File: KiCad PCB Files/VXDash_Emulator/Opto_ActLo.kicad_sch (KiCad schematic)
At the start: 3 parts

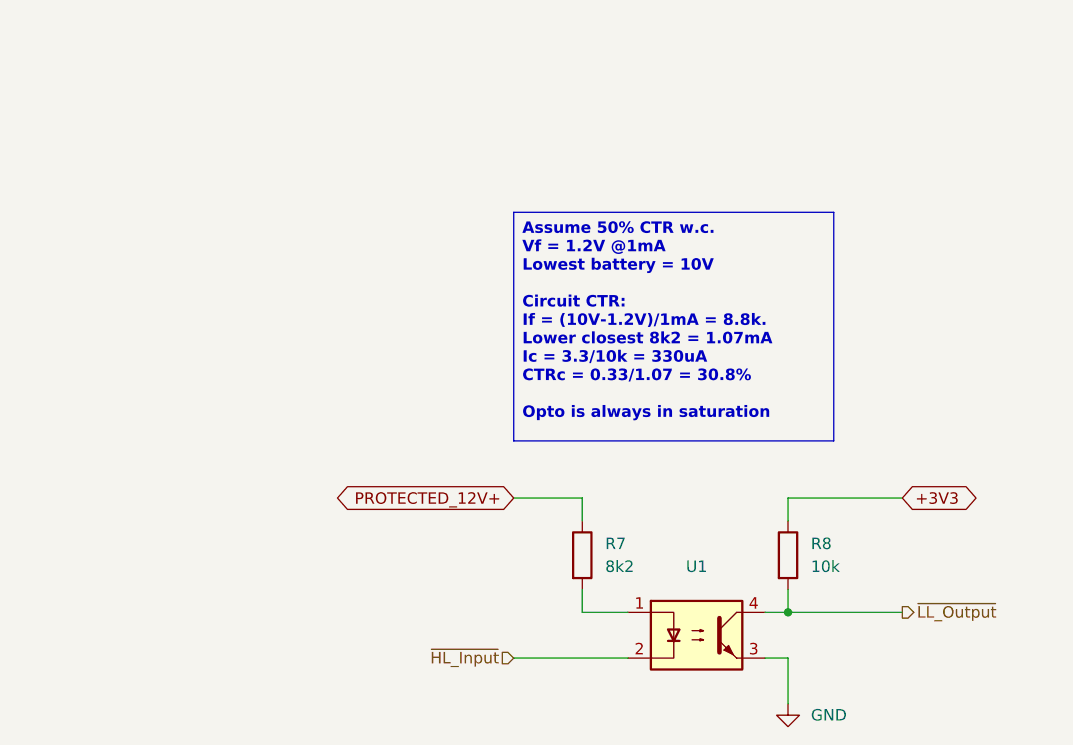
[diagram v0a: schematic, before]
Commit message: Emulator board refinements
- Is there stupid with the Active Hi Optos so that the logic is not inverted ?
- Added N-Mosfet activatable resistors. Stupidly simple ? Better MOSFET recommendation ?
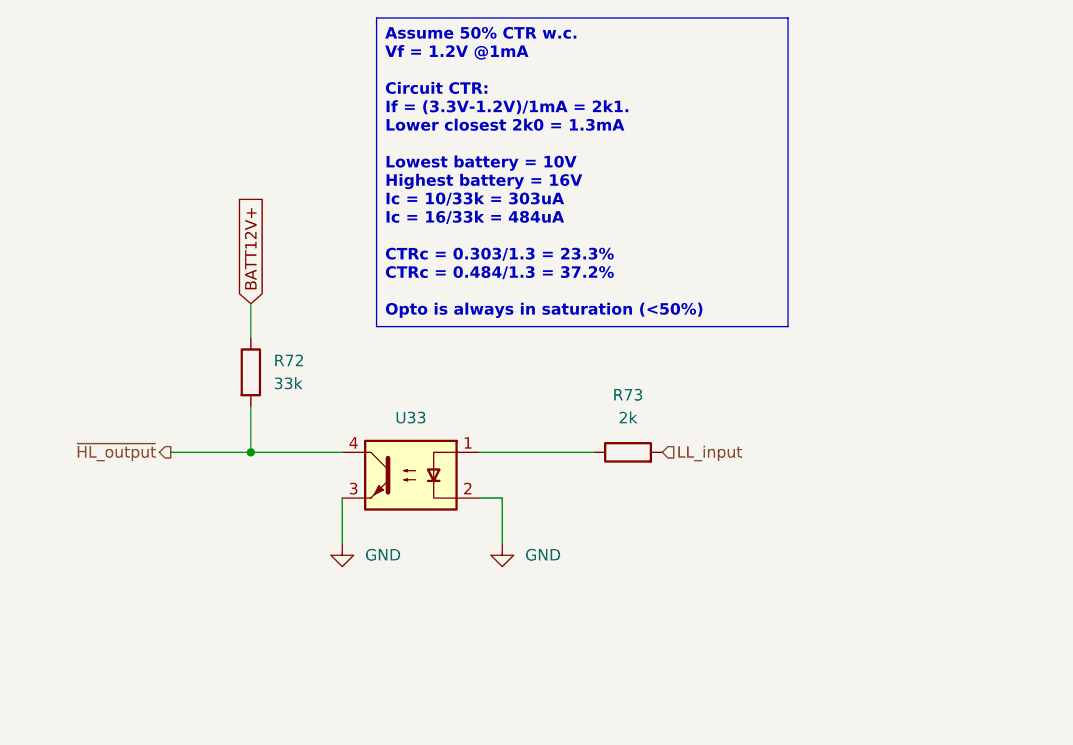
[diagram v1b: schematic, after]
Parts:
- removed R7: 8k2, Resistor_SMD:R_0805_2012Metric_Pad1.20x1.40mm_HandSolder, symbol VXDash_passives:Res
- removed R8: 10k, Resistor_SMD:R_0805_2012Metric_Pad1.20x1.40mm_HandSolder, symbol VXDash_passives:Res
- removed U1: ~, Package_DIP:SMDIP-4_W7.62mm, symbol Isolator:SFH617A-2X009T
- added R72: 33k, Resistor_SMD:R_0805_2012Metric_Pad1.20x1.40mm_HandSolder, symbol VXDash_passives:Res
- added R73: 2k, Resistor_SMD:R_0805_2012Metric_Pad1.20x1.40mm_HandSolder, symbol VXDash_passives:Res
- added U33: ~, Package_DIP:SMDIP-4_W7.62mm, symbol Isolator:SFH617A-2X009T
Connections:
- net GND: now also U33.2, U33.3
- new net: R73.1, U33.1
- new net BATT12V+: R72.1
- new net LL_input: R73.2
- new net ~{HL_output}: R72.2, U33.4
